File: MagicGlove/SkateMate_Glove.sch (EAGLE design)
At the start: 40 parts, among them IC1 BU33TD3WG, U1 ATMEGA328P-AU, Y1 8MHz

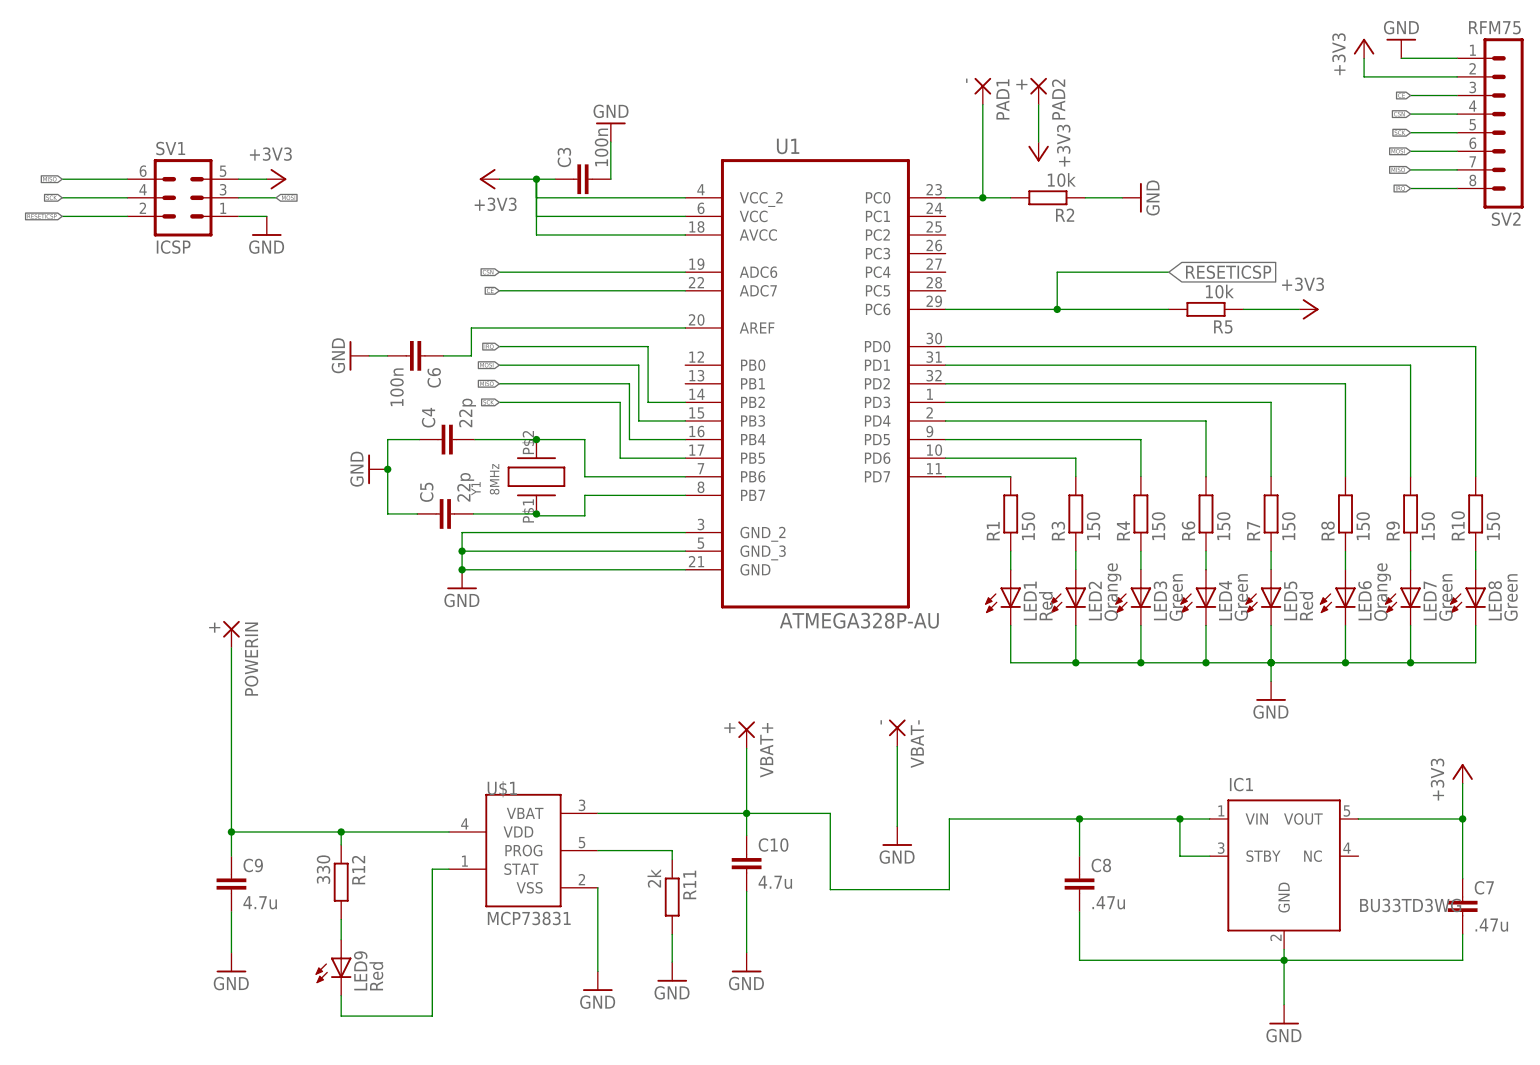
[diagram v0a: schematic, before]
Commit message: V0.9 Layout and Schematic ready for review and version jump to 1.0.
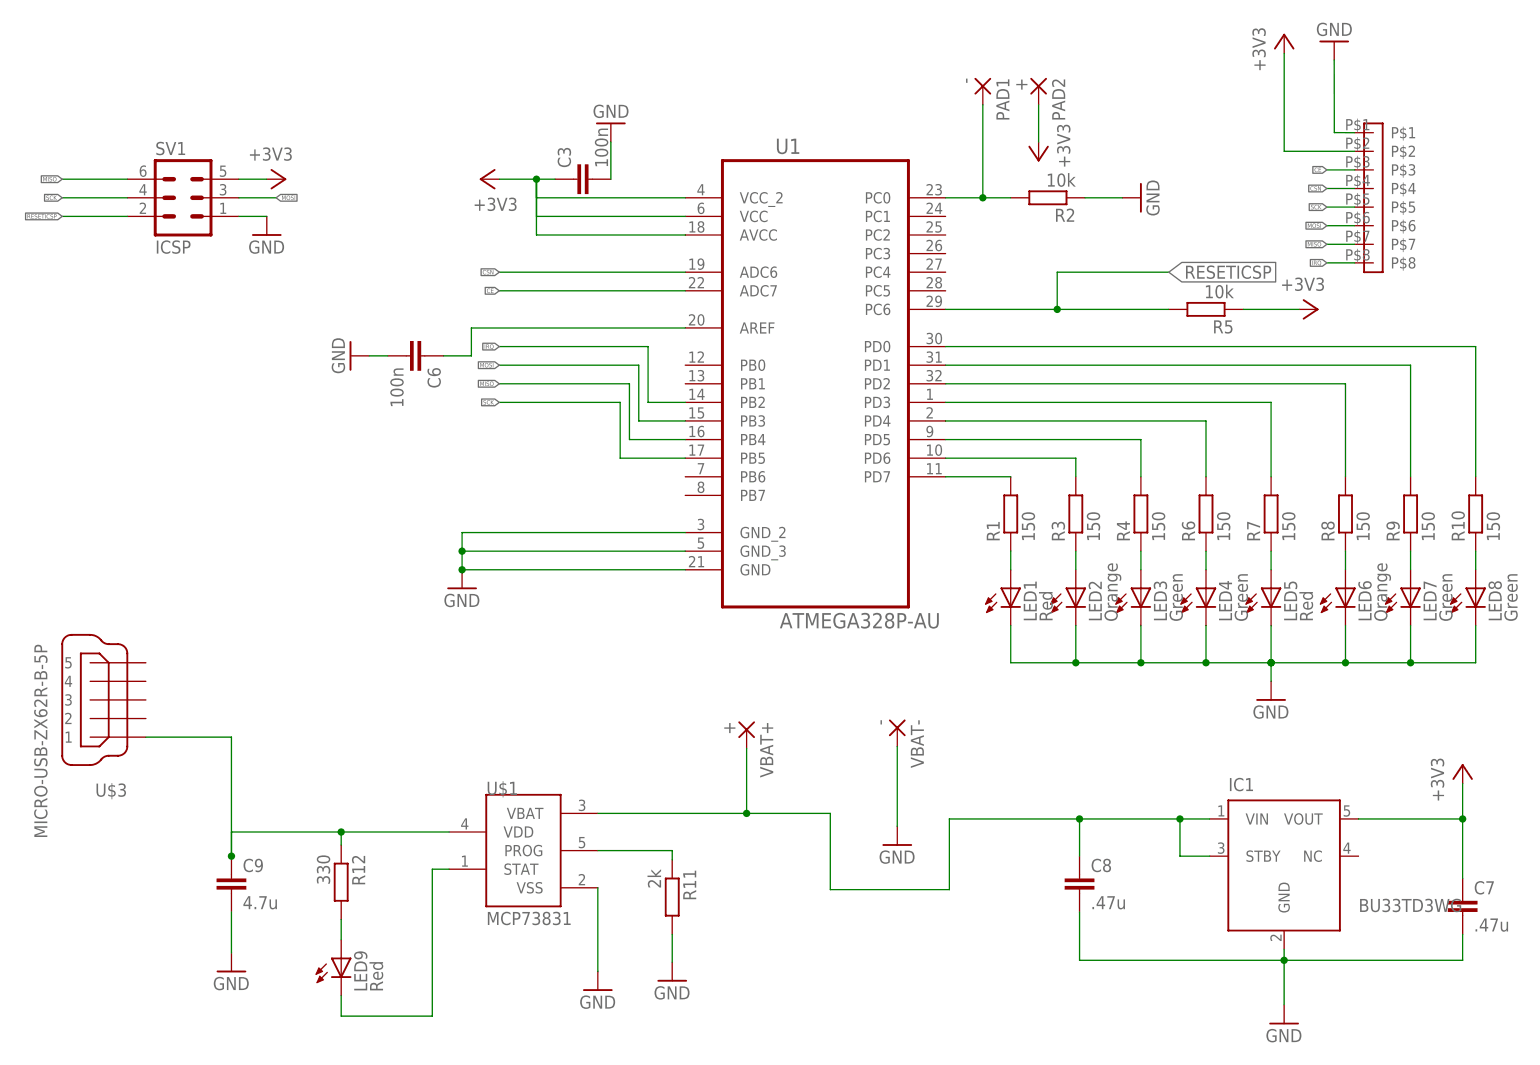
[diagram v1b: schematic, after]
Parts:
- removed C10: 4.7u, eagle-ltspice:CC0603
- removed C4, C5: 22p, eagle-ltspice:CC0603
- removed POWERIN: +, wirepad:1,6/0,8
- removed SV2: RFM75, con-lstb:MA08-1
- removed Y1: 8MHz, crystals:ABM3
- added U$2: HEADER1,27, SkateMateMagicGlove:HEADER1,27
- added U$3: MICRO-USB-ZX62R-B-5P, con-hirose:MICRO-USB-ZX62R-B-5P
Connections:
- removed net N$3: C5.2, U1.PB7, Y1.1
- removed net N$4: C4.2, U1.PB6, Y1.2
- net +3V3: now also U$2.P$2; no longer SV2.2
- net CE: now also U$2.P$3; no longer SV2.3
- net CSN: now also U$2.P$4; no longer SV2.4
- net GND: now also U$2.P$1; no longer C10.2, C4.1, C5.1, SV2.1
- net IRQ: now also U$2.P$8; no longer SV2.8
- net MISO: now also U$2.P$7; no longer SV2.7
- net MOSI: now also U$2.P$6; no longer SV2.6
- net N$21: no longer C10.1
- net N$24: now also U$3.1; no longer POWERIN.P
- net SCK: now also U$2.P$5; no longer SV2.5

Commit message: Revert "V0.9 Layout and Schematic ready for review and version jump to 1.0."
This reverts commit 28fefd69818988460ab9c4da467096be04e20f85.
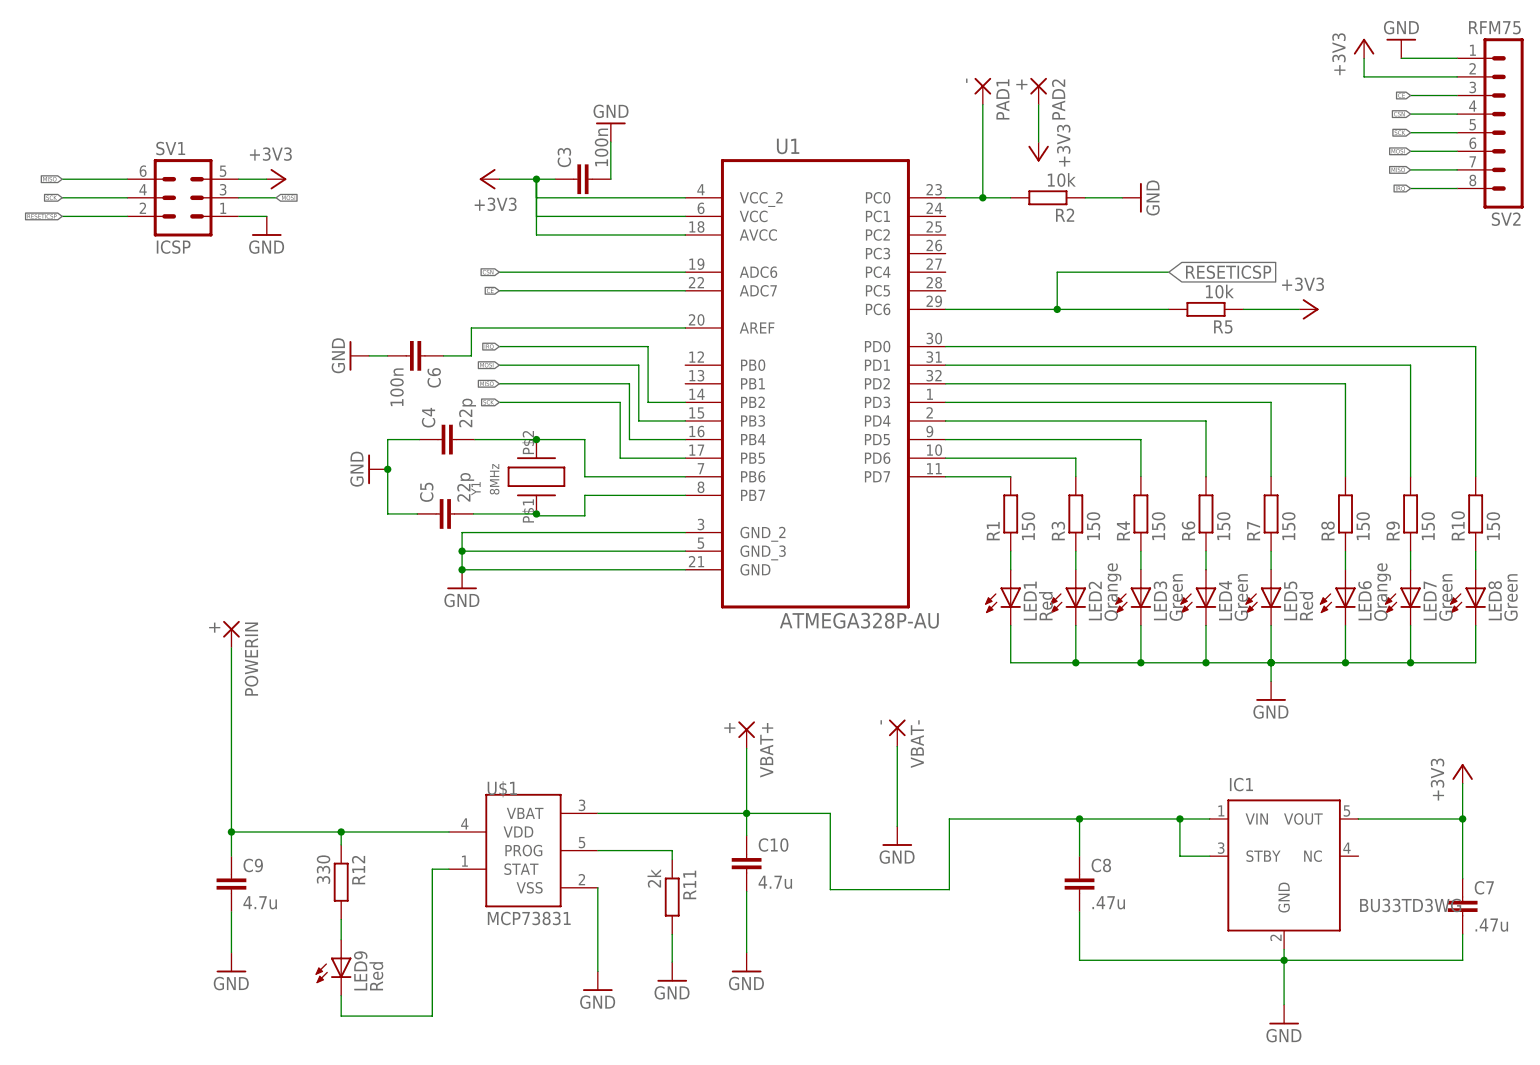
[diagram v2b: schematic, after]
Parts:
- removed U$2: HEADER1,27, SkateMateMagicGlove:HEADER1,27
- removed U$3: MICRO-USB-ZX62R-B-5P, con-hirose:MICRO-USB-ZX62R-B-5P
- added C10: 4.7u, eagle-ltspice:CC0603
- added C4, C5: 22p, eagle-ltspice:CC0603
- added POWERIN: +, wirepad:1,6/0,8
- added SV2: RFM75, con-lstb:MA08-1
- added Y1: 8MHz, crystals:ABM3
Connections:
- new net N$3: C5.2, U1.PB7, Y1.1
- new net N$4: C4.2, U1.PB6, Y1.2
- net +3V3: now also SV2.2; no longer U$2.P$2
- net CE: now also SV2.3; no longer U$2.P$3
- net CSN: now also SV2.4; no longer U$2.P$4
- net GND: now also C10.2, C4.1, C5.1, SV2.1; no longer U$2.P$1
- net IRQ: now also SV2.8; no longer U$2.P$8
- net MISO: now also SV2.7; no longer U$2.P$7
- net MOSI: now also SV2.6; no longer U$2.P$6
- net N$21: now also C10.1
- net N$24: now also POWERIN.P; no longer U$3.1
- net SCK: now also SV2.5; no longer U$2.P$5
